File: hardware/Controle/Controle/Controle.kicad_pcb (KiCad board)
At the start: 2 copper layers, 70 x 50 mm, 81 parts, among them J101 USART, J102 ST_LINK, J103 FAN, J105 Iin_sen, J106 Iin_sen, J107 Driver-Sense, J301 RJ45, Q101 BCV27, U201 MCP2561-E-SN, U401 AMS1117-3.3, U402 AMS1117-5, U403 K78L15-1000R3, U501 STM32G431CBT6, U601 TL7726IDR

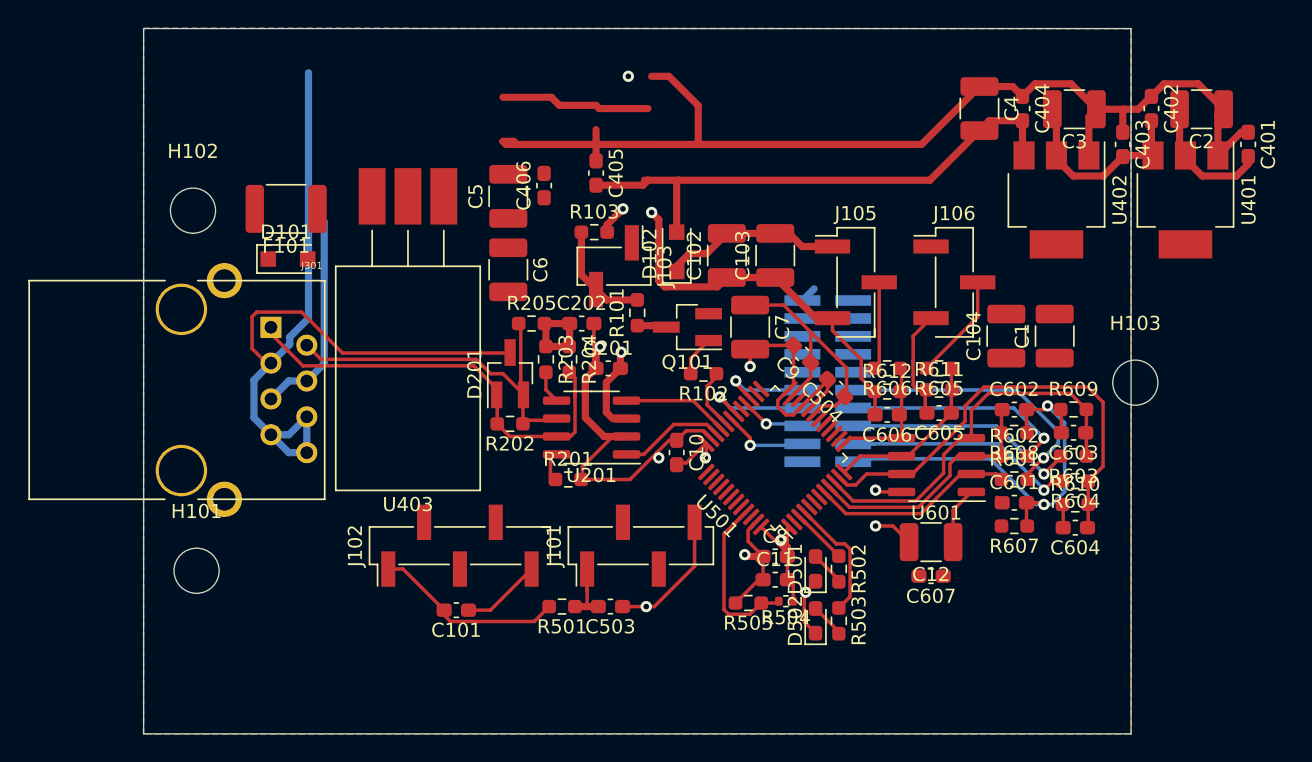
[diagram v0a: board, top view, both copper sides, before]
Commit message: falta acabamento
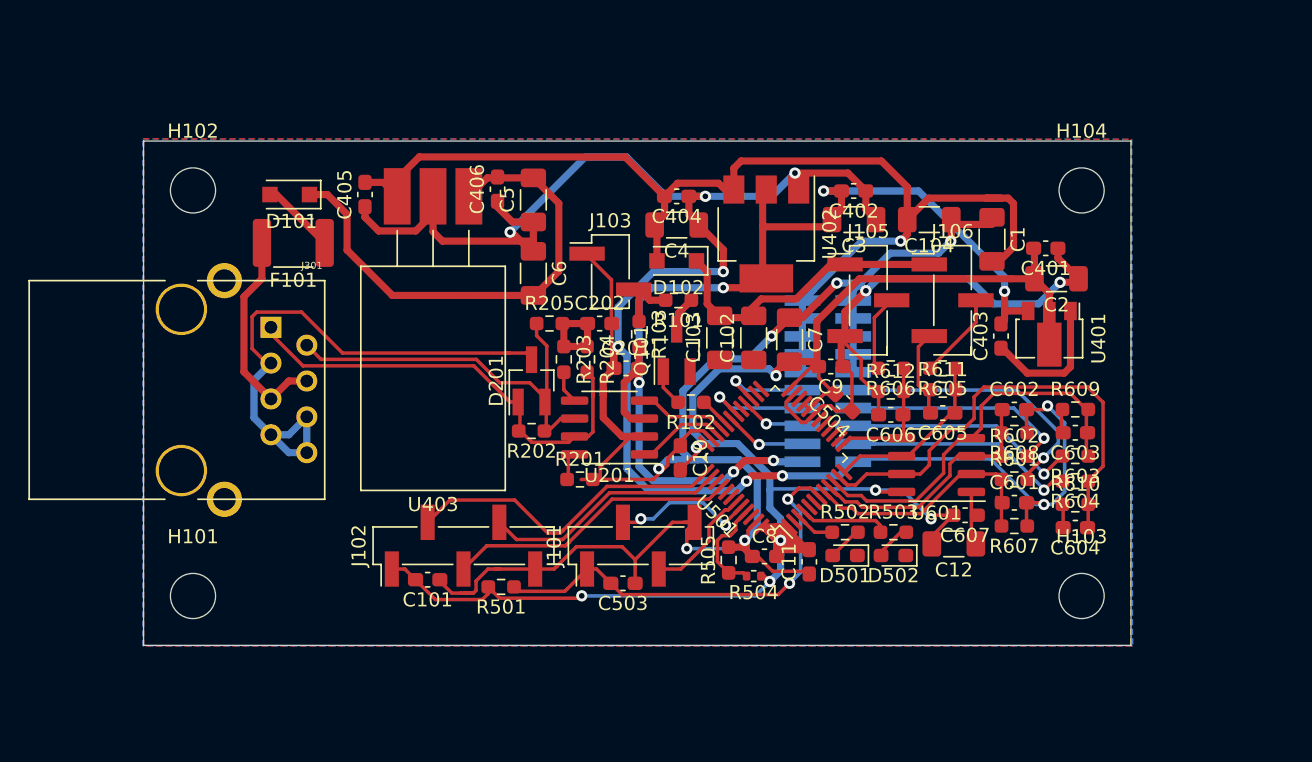
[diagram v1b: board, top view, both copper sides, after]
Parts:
- added H104: MountingHole, MountingHole:MountingHole_3.2mm_M3, F.Cu at (192.2, 57.0)
- C1, C102, C103, C104, C12, C2, C3, C4, C5, C6, C7: footprint Capacitor_SMD:C_1210_3225Metric_Pad1.33x2.70mm_HandSolder -> Capacitor_SMD:C_1206_3216Metric_Pad1.33x1.80mm_HandSolder
- U401: footprint Package_TO_SOT_SMD:SOT-223-3_TabPin2 -> Package_TO_SOT_SMD:SOT-89-3
- moved C404 25.3 mm to (163.5, 57.4), turned to 180 degrees
- moved C4 23.0 mm to (163.5, 59.4), turned to 180 degrees
- moved C402 21.9 mm to (176.1, 57.0), turned to 180 degrees
- moved U402 20.7 mm to (169.9, 60.1)
- moved C3 17.5 mm to (176.1, 59.0)
- moved C405 16.5 mm to (141.4, 57.3), turned to 90 degrees
- moved C401 16.1 mm to (189.7, 61.1), turned to 180 degrees
- moved C403 16.1 mm to (186.5, 67.3), turned to 90 degrees
- moved C2 15.8 mm to (190.4, 63.2)
- moved H103 15.6 mm to (192.2, 85.7)
- moved U401 13.6 mm to (189.9, 67.2)
- moved C104 9.90 mm to (181.4, 59.0), turned to 180 degrees
- moved C1 8.17 mm to (185.9, 60.4), turned to 270 degrees
- moved R103 7.90 mm to (160.8, 67.2), turned to 270 degrees
- moved R503 7.38 mm to (178.9, 81.2), turned to 0 degrees
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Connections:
- J102 pad 2: /STM32/SWCLK -> /STM32/SWDIO
- J102 pad 3: /STM32/SWDIO -> /STM32/SWO
- J102 pad 4: /STM32/SWO -> /STM32/SWCLK
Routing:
- net GND: track 286.6 -> 370.8 mm, vias 9 -> 17
- net +3V3: track 60.1 -> 138.3 mm, vias 5 -> 7
- net +5V: track 23.4 -> 77.7 mm, vias 2 -> 6
- net +15V: track 40.0 -> 83.4 mm, vias 0 -> 1
- net /STM32/RESET: track 6.37 -> 32.7 mm, vias 0 -> 2
- net /Powersupply/+18V: track 10.6 -> 35.4 mm
- net /STM32/SWDIO: track 0.00 -> 23.3 mm
- net /STM32/SWO: track 0.00 -> 20.9 mm
- net /STM32/SWCLK: track 0.00 -> 17.4 mm
- net /STM32/USART3_RX: track 0.00 -> 10.3 mm, vias 0 -> 2
- net Net-(C102-Pad2): track 12.9 -> 21.6 mm
- net /STM32/USART3_TX: track 0.00 -> 8.60 mm
- net Net-(D101-Pad2): track 0.00 -> 5.30 mm
- net /STM32/BOOT0: track 13.1 -> 7.99 mm
- net Net-(J103-Pad2): track 7.72 -> 4.20 mm
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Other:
- board size 70 x 50 mm -> 70 x 35.8 mm
